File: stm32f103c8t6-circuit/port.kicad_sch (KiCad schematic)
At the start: 26 parts, among them J1 Conn_01x04, J1 Conn_01x06, J3 Conn_01x03, J4 Conn_01x02, J4 Conn_01x03, J5 Conn_01x03, J5 USB_C_Receptacle_USB2.0, J6 Conn_01x04, J8 Conn_01x02, SW2 , SW3 , U4 TJA1051T-3, U5 CH340E

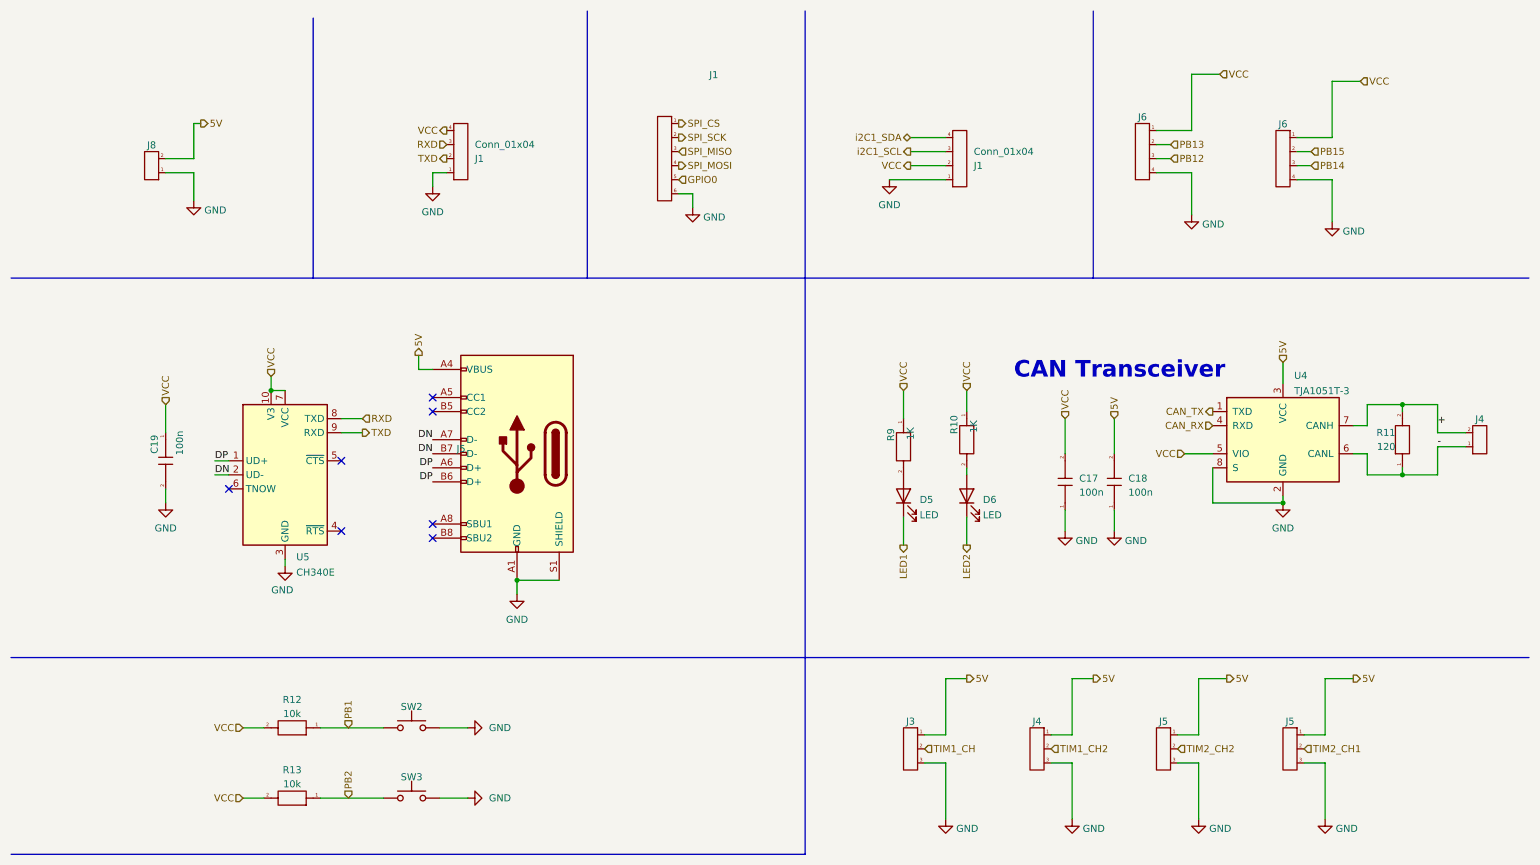
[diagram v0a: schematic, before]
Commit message: Modify PCH and SCH
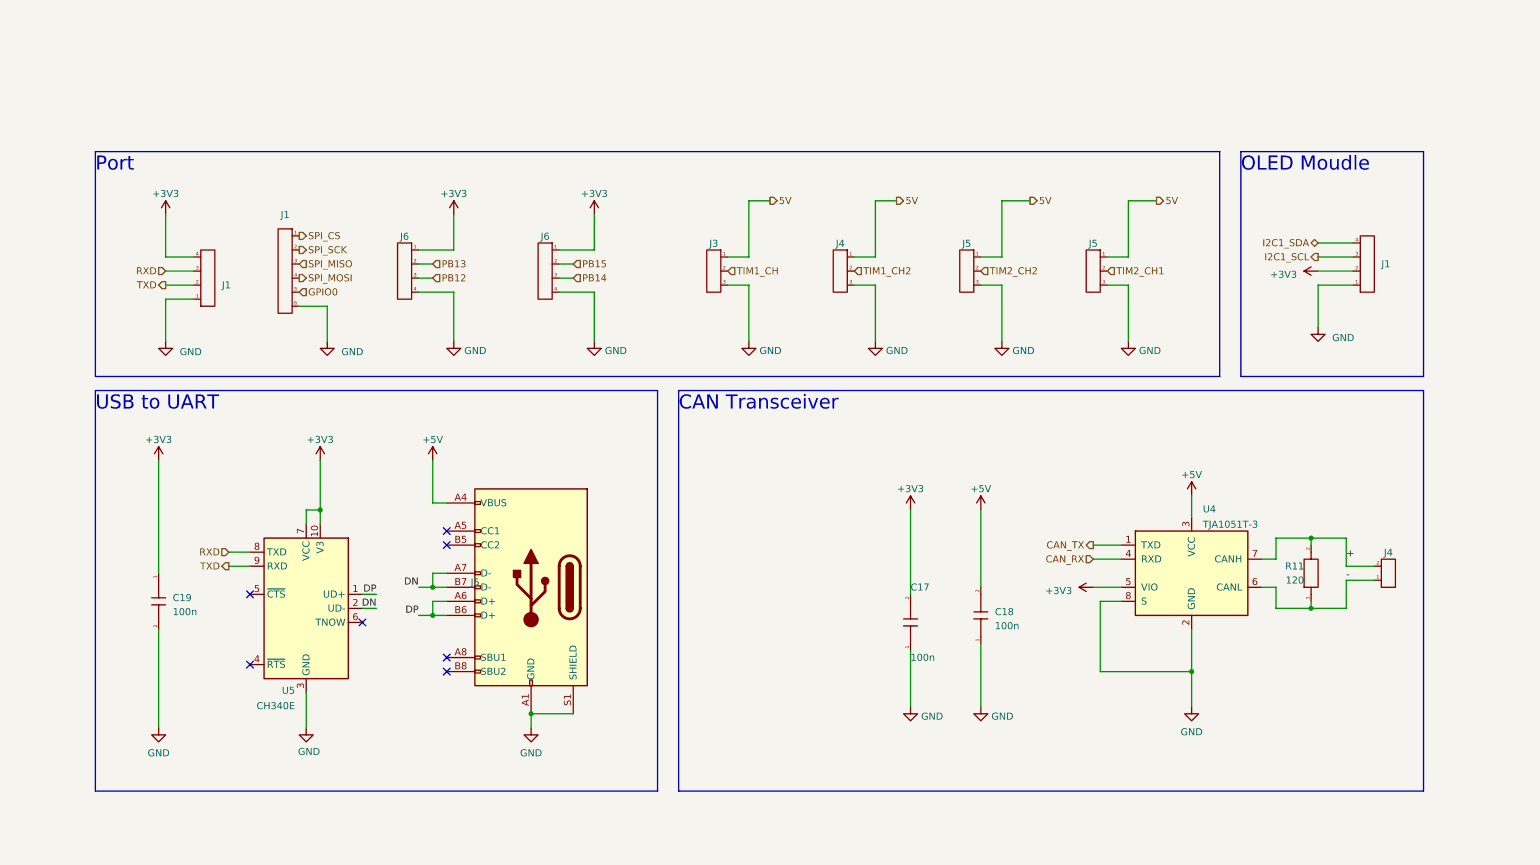
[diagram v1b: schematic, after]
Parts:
- removed D5, D6: LED, LED_SMD:LED_0603_1608Metric, symbol Device:LED
- removed J8: Conn_01x02, Connector_AMASS:AMASS_XT30UPB-M_1x02_P5.0mm_Vertical, symbol 302_Link_W2B-Connector:Conn_01x02
- removed R10, R9: 1K, PCM_001_GN_RCL_SMD:R0603(1608M), symbol 001_Basic_PassiveComponents:001_Resistor
- removed R12, R13: 10k, PCM_001_GN_RCL_SMD:R0603(1608M), symbol 001_Basic_PassiveComponents:001_Resistor
- removed SW2, SW3: (no value), Button_Switch_SMD:SW_SPST_FSMSM, symbol Switch:SW_Push
- J1: footprint PCM_205_CONN_GH_SMD:GH1.25_H_4 -> Connector_PinHeader_2.54mm:PinHeader_1x04_P2.54mm_Vertical
- R11: footprint PCM_001_GN_RCL_SMD:R0603(1608M) -> ResistorSMD:R_0603_1608Metric
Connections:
- net 5V: no longer C18.2, J5.A4 (VBUS), J5.A9 (VBUS), J5.B4 (VBUS), J5.B9 (VBUS), U4.3 (VCC)
- net VCC renamed +3V3
- net i2C1_SCL renamed I2C1_SCL
- net i2C1_SDA renamed I2C1_SDA
- new net +5V: C18.2, J5.A4 (VBUS), J5.A9 (VBUS), J5.B4 (VBUS), J5.B9 (VBUS), U4.3 (VCC)
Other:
- note added: "OLED Moudle"
- note added: "Port"
- note added: "USB to UART"
- moved on the sheet: C17, C18, C19, J1, J3, J4, J5, J6, R11, U4, U5
